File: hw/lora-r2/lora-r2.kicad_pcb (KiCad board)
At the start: 2 copper layers, 74 x 59 mm, 18 parts, among them J1 Conn_Coaxial, J2 SWD, J3 Conn_02x08_Odd_Even, J4 Conn_01x06, Q1 IRLML6401, U1 Pico_1_PCB, U3 MCP1700x-330xxTT

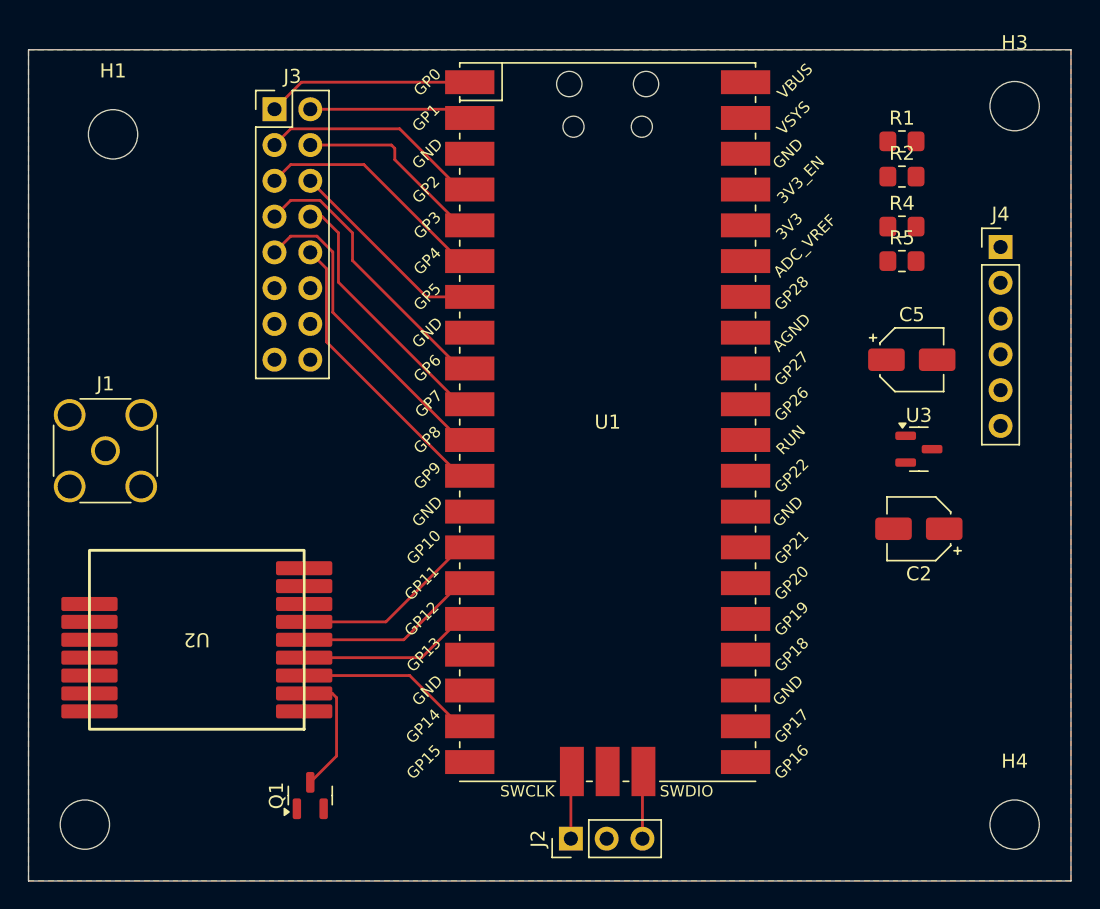
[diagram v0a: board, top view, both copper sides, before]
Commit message: Making progress on layout
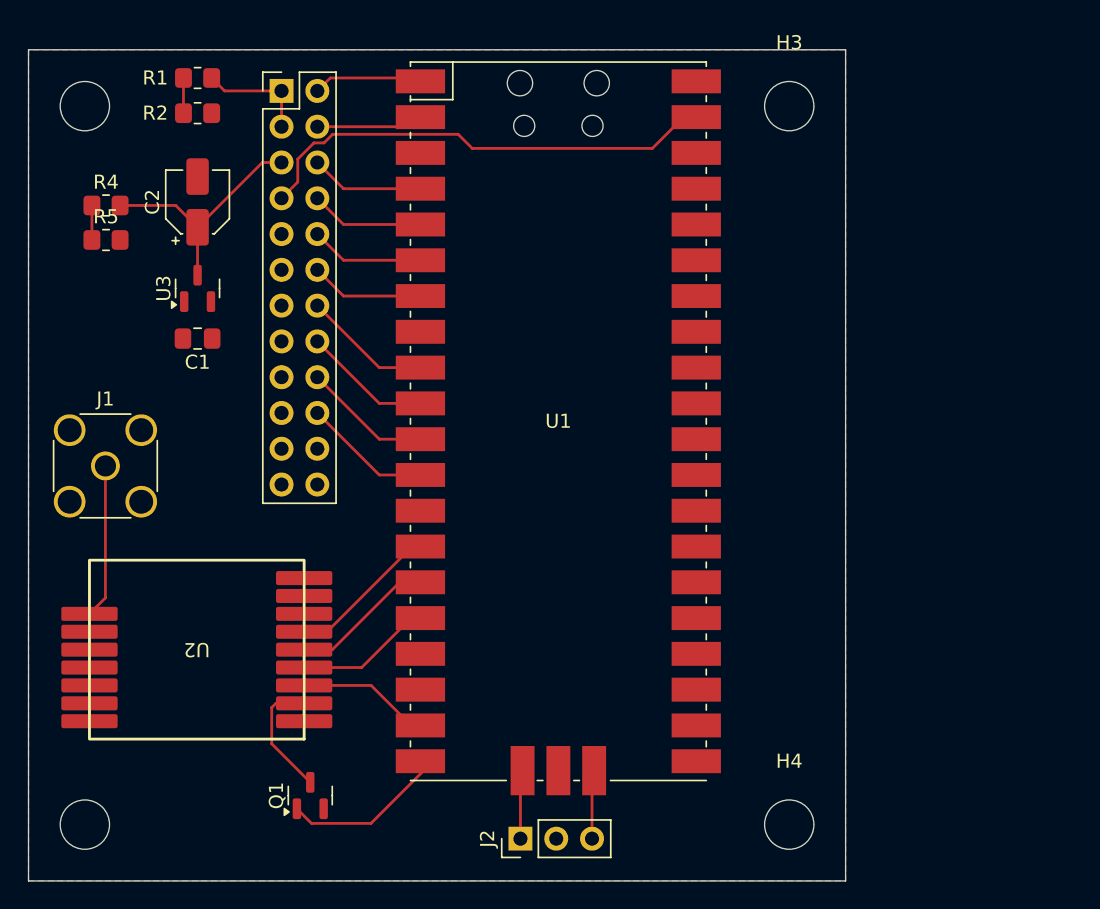
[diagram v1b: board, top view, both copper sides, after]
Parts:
- removed C5: 10u, Capacitor_SMD:CP_Elec_4x5.4
- removed J4: Conn_01x06, Connector_PinHeader_2.54mm:PinHeader_1x06_P2.54mm_Vertical
- added C1: 10u, Capacitor_SMD:C_0805_2012Metric_Pad1.18x1.45mm_HandSolder, F.Cu at (80.0, 97.5)
- J3: value Conn_02x08_Odd_Even -> Conn_02x12_Odd_Even; footprint Connector_PinHeader_2.54mm:PinHeader_2x08_P2.54mm_Vertical -> Connector_PinHeader_2.54mm:PinHeader_2x12_P2.54mm_Vertical
- moved R4 56.5 mm to (73.5, 88.0)
- moved R5 56.5 mm to (73.5, 90.5)
- moved C2 56.2 mm to (80.0, 87.8), turned to 90 degrees
- moved U3 52.5 mm to (80.0, 93.9), turned to 90 degrees
- moved R1 50.2 mm to (80.0, 79.0)
- moved R2 50.2 mm to (80.0, 81.5)
- moved H3 16.0 mm to (122.0, 81.0)
- moved H4 16.0 mm to (122.0, 132.0)
- moved J2 3.58 mm to (102.9, 133.0)
- moved U1 3.50 mm to (105.6, 103.4)
- moved H1 2.83 mm to (72.0, 81.0)
- moved J3 1.39 mm to (86.0, 79.9)
- moved J1 1.08 mm to (73.5, 106.5)
- moved U2 0.70 mm to (87.6, 124.7)
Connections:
- C2 pad 1: VCONV -> VCON
- J3 pad 1: GPIO0 -> VPAN
- J3 pad 10: GPIO9 -> GPIO4
- J3 pad 11: VPAN_SENSE -> VCON_SENSE
- J3 pad 12: GPIO26 -> GPIO5
- J3 pad 13: VCON_SENSE -> GPIO27
- J3 pad 14: GPIO27 -> GPIO6
- J3 pad 15: GND -> VPAN_SENSE
- J3 pad 16: GND -> GPIO7
- J3 pad 2: GPIO1 -> GPIO0
- J3 pad 3: GPIO2 -> VPAN
- J3 pad 4: GPIO3 -> GPIO1
- J3 pad 5: GPIO4 -> VCON
- J3 pad 6: GPIO5 -> GPIO2
- J3 pad 7: GPIO6 -> +3.3V
- J3 pad 8: GPIO7 -> GPIO3
- J3 pad 9: GPIO8 -> GPIO26
- Q1 pad 1: GPIO20 -> GPIO15
- U1 pad 20: unconnected-(U1-GPIO15-Pad20) -> GPIO15
- U1 pad 26: GPIO20 -> unconnected-(U1-GPIO20-Pad26)
- U3 pad 2: +3V3 -> +3.3V
- U3 pad 3: VCONV -> VCON
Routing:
- net +3.3V: track 0.00 -> 32.7 mm
- net VCON: track 0.00 -> 17.5 mm
- net GPIO8: track 23.7 -> 10.0 mm
- net GPIO15: track 0.00 -> 11.9 mm
- net GPIO9: track 21.8 -> 10.0 mm
- net GPIO6: track 21.3 -> 10.0 mm
- net Net-(J1-In): track 0.00 -> 11.0 mm
- net GPIO7: track 19.8 -> 10.0 mm
- net GPIO4: track 18.1 -> 8.99 mm
- net GPIO2: track 17.0 -> 8.99 mm
- net VPAN: track 0.00 -> 7.88 mm
- net GPIO0: track 15.6 -> 8.70 mm
- net GPIO5: track 15.6 -> 8.99 mm
- net GPIO3: track 15.1 -> 8.99 mm
- net GPIO1: track 12.5 -> 8.50 mm
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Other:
- board size 74 x 59 mm -> 58 x 59 mm
